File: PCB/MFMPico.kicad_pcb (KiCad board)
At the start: 2 copper layers, 96.5 x 96 mm, 29 parts, among them J1 ECON34, J2 Conn_02x04_Odd_Even, J3 Micro_SD_Card, J4 Conn_01x16, J5 Conn_01x04, J6 Conn_01x02, J7 Conn_01x02, P1 CON20, U2 74LS03, U3 74LS03, U4 74LS03, U5 SN65HVD33DR

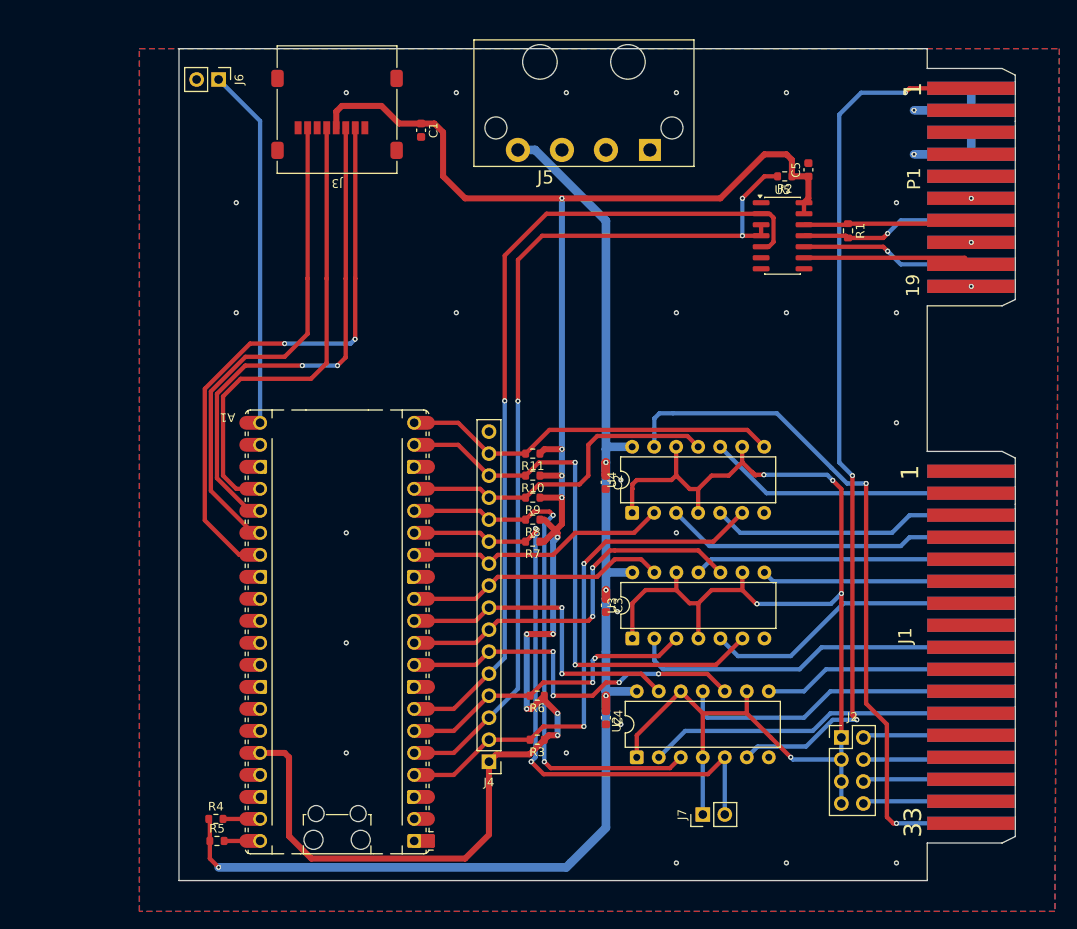
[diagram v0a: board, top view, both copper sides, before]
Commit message: Mostly up to date PCB
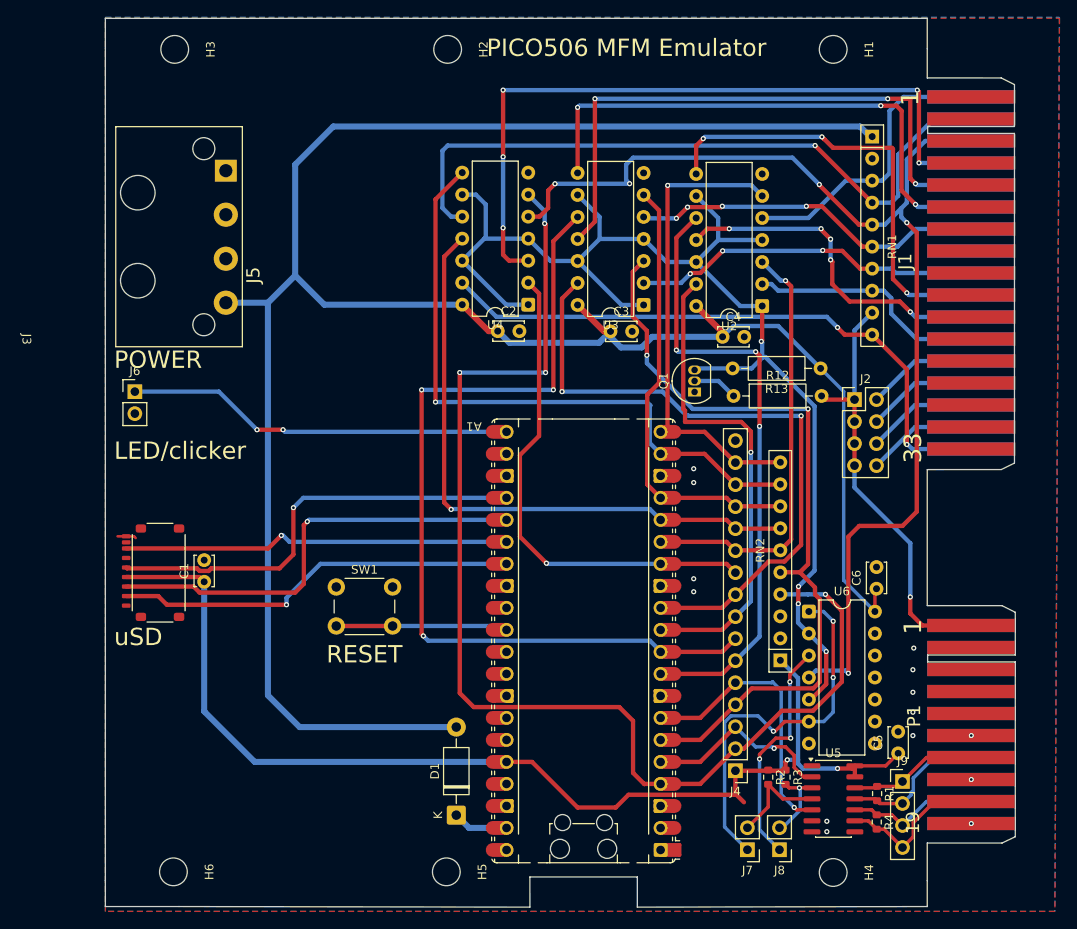
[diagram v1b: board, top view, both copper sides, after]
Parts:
- removed R10, R11, R6, R7, R8, R9: 1K, Resistor_SMD:R_0603_1608Metric
- removed R5: R, Resistor_SMD:R_0603_1608Metric
- added C6: 100n, Capacitor_THT:C_Disc_D3.4mm_W2.1mm_P2.50mm, F.Cu at (175.5, 120.8)
- added D1: 1N5818, Diode_THT:D_DO-41_SOD81_P10.16mm_Horizontal, F.Cu at (127.0, 146.9)
- added H1: MountingHole, MountingHole:MountingHole_3.2mm_M3, F.Cu at (170.5, 58.5)
- added H2: MountingHole, MountingHole:MountingHole_3.2mm_M3, F.Cu at (126.0, 58.5)
- added H3: MountingHole, MountingHole:MountingHole_3.2mm_M3, F.Cu at (94.5, 58.5)
- added H4: MountingHole, MountingHole:MountingHole_3.2mm_M3, F.Cu at (170.5, 153.5)
- added H5: MountingHole, MountingHole:MountingHole_3.2mm_M3, F.Cu at (125.8, 153.4)
- added H6: MountingHole, MountingHole:MountingHole_3.2mm_M3, F.Cu at (94.3, 153.4)
- added J8: Conn_01x02, Connector_PinHeader_2.54mm:PinHeader_1x02_P2.54mm_Vertical, F.Cu at (164.3, 150.9)
- added J9: Conn_01x04, Connector_PinHeader_2.54mm:PinHeader_1x04_P2.54mm_Vertical, F.Cu at (178.5, 143.0)
- added Q1: BC547, Package_TO_SOT_THT:TO-92_Inline, F.Cu at (154.5, 98.0)
- added R12: 5.1K, Resistor_THT:R_Axial_DIN0207_L6.3mm_D2.5mm_P10.16mm_Horizontal, F.Cu at (159.0, 98.5)
- added R13: 220R, Resistor_THT:R_Axial_DIN0207_L6.3mm_D2.5mm_P10.16mm_Horizontal, F.Cu at (169.1, 95.3)
- added RN1: R_Network09, Resistor_THT:R_Array_SIP10, F.Cu at (175.0, 68.6)
- added RN2: R_Network09, Resistor_THT:R_Array_SIP10, F.Cu at (164.4, 129.0)
- added SW1: SW_Push, Button_Switch_THT:SW_PUSH_6mm, F.Cu at (113.2, 120.5)
- added U6: 74LS03, Package_DIP:DIP-14_W7.62mm, F.Cu at (167.7, 123.4)
- C1, C2, C3, C4, C5: footprint Capacitor_SMD:C_0603_1608Metric -> Capacitor_THT:C_Disc_D3.4mm_W2.1mm_P2.50mm
- J3: footprint Connector_Card:microSD_HC_Molex_47219-2001 -> rik:microSD Hanbo Electronic TF-018
- R2: value 5.1K -> 470R
- R3: value 1K -> 470R
- R4: value R -> 100R
- moved R4 76.3 mm to (175.5, 147.7), turned to -90 degrees
- moved R2 69.4 mm to (163.0, 142.5), turned to -90 degrees
- moved C5 68.1 mm to (178.0, 139.8)
- moved U5 65.3 mm to (170.5, 145.0)
- moved R1 65.0 mm to (175.6, 144.4)
- moved J3 62.2 mm to (88.9, 122.7), turned to -90 degrees
- moved P1 62.0 mm to (186.2, 135.1)
- moved C1 57.8 mm to (97.9, 120.0), turned to 90 degrees
- moved U2 54.1 mm to (162.3, 88.1), turned to 180 degrees
- moved C4 46.0 mm to (157.7, 91.7), turned to 0 degrees
- moved J1 43.2 mm to (180.1, 83.0)
- moved J2 39.0 mm to (173.0, 98.9)
- moved U3 38.5 mm to (148.6, 88.0), turned to 180 degrees
- moved J5 37.7 mm to (105.5, 78.8), turned to 90 degrees
- moved J6 37.3 mm to (89.9, 98.0), turned to 0 degrees
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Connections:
- net Net-(J1-Write_gate) renamed /~WRITE_GATE
- A1 pad 15: /SELECT -> /STEP
- A1 pad 16: /STEP -> /DIR_IN
- A1 pad 17: /DIR_IN -> /HEAD_0
- A1 pad 19: /HEAD_0 -> /HEAD_2
- A1 pad 20: /HEAD_2 -> /HEAD_3
- A1 pad 30: unconnected-(A1-RUN-Pad30) -> Net-(A1-RUN)
- A1 pad 40: Net-(A1-VBUS) -> unconnected-(A1-VBUS-Pad40)
- J1 pad 2: unconnected-(J1-Head_3/REDWR-Pad2) -> Net-(J1-Head_3/REDWR)
- J2 pad 1: /DRIVE_SEL -> /~DRIVE_SEL
- J2 pad 3: /DRIVE_SEL -> /~DRIVE_SEL
- J2 pad 5: /DRIVE_SEL -> /~DRIVE_SEL
- J2 pad 7: /DRIVE_SEL -> /~DRIVE_SEL
- J4 pad 11: /SELECT -> /STEP
- J4 pad 12: /STEP -> /DIR_IN
- J4 pad 13: /DIR_IN -> /HEAD_0
- J4 pad 14: /HEAD_0 -> /HEAD_2
- J4 pad 15: /HEAD_2 -> /HEAD_3
- J7 pad 1: /DRIVE_SEL -> Net-(J7-Pin_1)
- J7 pad 2: /SELECT -> Net-(J7-Pin_2)
- P1 pad 1: Net-(P1-Drive_Selected) -> /~DRIVE_SEL
- P1 pad 17: Net-(P1-MFM_Read+) -> Net-(J9-Pin_4)
- P1 pad 18: Net-(P1-MFM_Read-) -> Net-(J9-Pin_3)
- R2 pad 2: /MFM_IN -> Net-(J7-Pin_2)
- R3 pad 2: /WRITE_GATE -> Net-(J8-Pin_2)
- R4 pad 1: +5V -> Net-(J9-Pin_3)
- R4 pad 2: Net-(A1-VSYS) -> Net-(J9-Pin_4)
- U2 pad 5: /SELECT -> Net-(J1-Head_3/REDWR)
- U2 pad 6: Net-(P1-Drive_Selected) -> /HEAD_3
- U5 pad 10: Net-(P1-MFM_Read-) -> Net-(J9-Pin_3)
- U5 pad 2: /MFM_OUT -> /MFM_IN
- U5 pad 3: /MFM_IN -> Net-(J8-Pin_2)
- U5 pad 4: /MFM_IN -> Net-(J7-Pin_2)
- U5 pad 9: Net-(P1-MFM_Read+) -> Net-(J9-Pin_4)
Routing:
- net +5V: track 150.3 -> 271.4 mm, vias 4 -> 0
- net /~WRITE_GATE: track 30.8 -> 132.8 mm, vias 0 -> 5
- net Net-(P1-Drive_Selected): track 101.7 -> 0.00 mm, vias 3 -> 0
- net /MFM_IN: track 103.7 -> 21.7 mm, vias 3 -> 1
- net +3.3V: track 212.1 -> 130.5 mm, vias 10 -> 2
- net /WRITE_GATE: track 60.6 -> 140.4 mm, vias 2 -> 4
- net /SELECT: track 72.0 -> 0.00 mm, vias 2 -> 0
- net /MFM_OUT: track 96.2 -> 31.5 mm
- net /WRITE_FAULT: track 43.3 -> 102.3 mm, vias 2 -> 3
- net /HEAD_3: track 0.00 -> 54.4 mm, vias 0 -> 1
- net /HEAD_1: track 35.4 -> 89.2 mm
- net /~DRIVE_SEL: track 0.00 -> 49.8 mm, vias 0 -> 1
- net Net-(J1-Head_2): track 31.2 -> 80.1 mm, vias 0 -> 1
- net Net-(J1-Seek_Complete): track 36.1 -> 84.5 mm, vias 0 -> 5
- net /TRACK_0: track 29.4 -> 75.4 mm, vias 0 -> 2
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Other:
- board size 96.5 x 96 mm -> 105 x 102.6 mm
- board text added: "LED/clicker"
- board text added: "PICO506 MFM Emulator"
- board text added: "POWER"
- board text added: "RESET"
- board text added: "uSD"
